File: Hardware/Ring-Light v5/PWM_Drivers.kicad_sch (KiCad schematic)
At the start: 39 parts, among them U33 PCA9685BS,118, U34 PCA9685BS,118

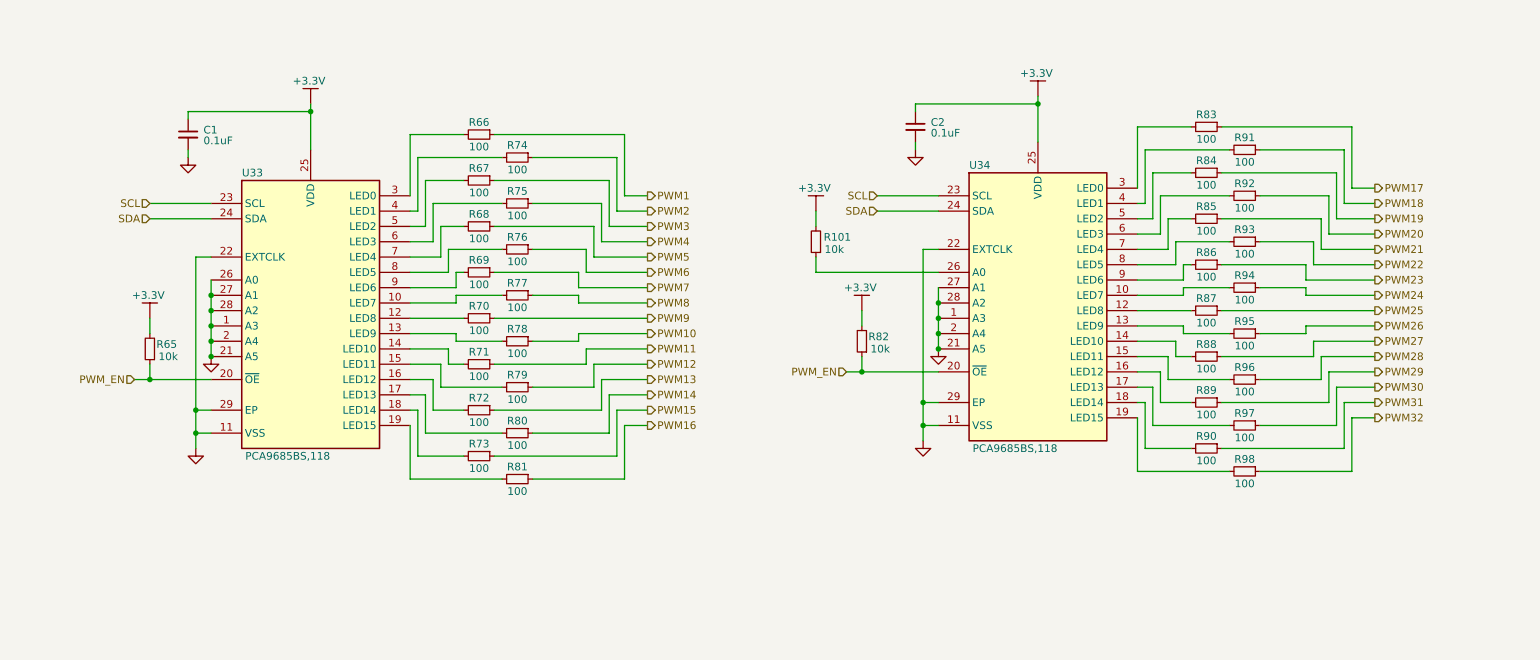
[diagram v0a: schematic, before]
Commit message: m
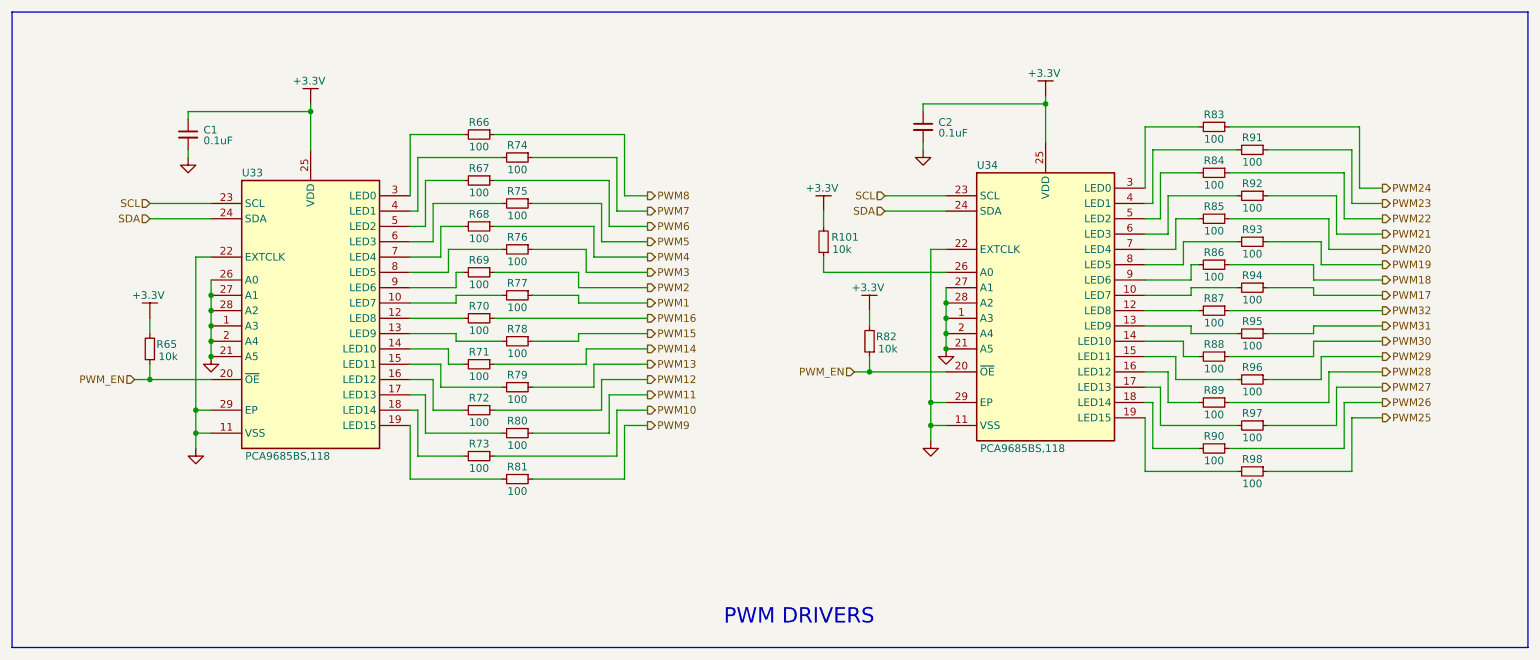
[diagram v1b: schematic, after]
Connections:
- net PWM1: now also R77.1; no longer R66.1
- net PWM10: now also R73.1; no longer R78.1
- net PWM11: now also R80.1; no longer R71.1
- net PWM12: now also R72.1; no longer R79.1
- net PWM13: now also R79.1; no longer R72.1
- net PWM14: now also R71.1; no longer R80.1
- net PWM15: now also R78.1; no longer R73.1
- net PWM16: now also R70.1; no longer R81.1
- net PWM17: now also R94.1; no longer R83.1
- net PWM18: now also R86.1; no longer R91.1
- net PWM19: now also R93.1; no longer R84.1
- net PWM2: now also R69.1; no longer R74.1
- net PWM20: now also R85.1; no longer R92.1
- net PWM21: now also R92.1; no longer R85.1
- net PWM22: now also R84.1; no longer R93.1
- net PWM23: now also R91.1; no longer R86.1
- net PWM24: now also R83.1; no longer R94.1
- net PWM25: now also R98.1; no longer R87.1
- net PWM26: now also R90.1; no longer R95.1
- net PWM27: now also R97.1; no longer R88.1
- net PWM28: now also R89.1; no longer R96.1
- net PWM29: now also R96.1; no longer R89.1
- net PWM3: now also R76.1; no longer R67.1
- net PWM30: now also R88.1; no longer R97.1
- net PWM31: now also R95.1; no longer R90.1
- net PWM32: now also R87.1; no longer R98.1
- net PWM4: now also R68.1; no longer R75.1
- net PWM5: now also R75.1; no longer R68.1
- net PWM6: now also R67.1; no longer R76.1
- net PWM7: now also R74.1; no longer R69.1
- net PWM8: now also R66.1; no longer R77.1
- net PWM9: now also R81.1; no longer R70.1
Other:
- note added: "PWM DRIVERS"
- moved on the sheet: C2, R101, R82, R83, R84, R85, R86, R87, R88, R89, R90, R91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
